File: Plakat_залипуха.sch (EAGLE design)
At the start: 25 parts, among them X1 USB-MICROB

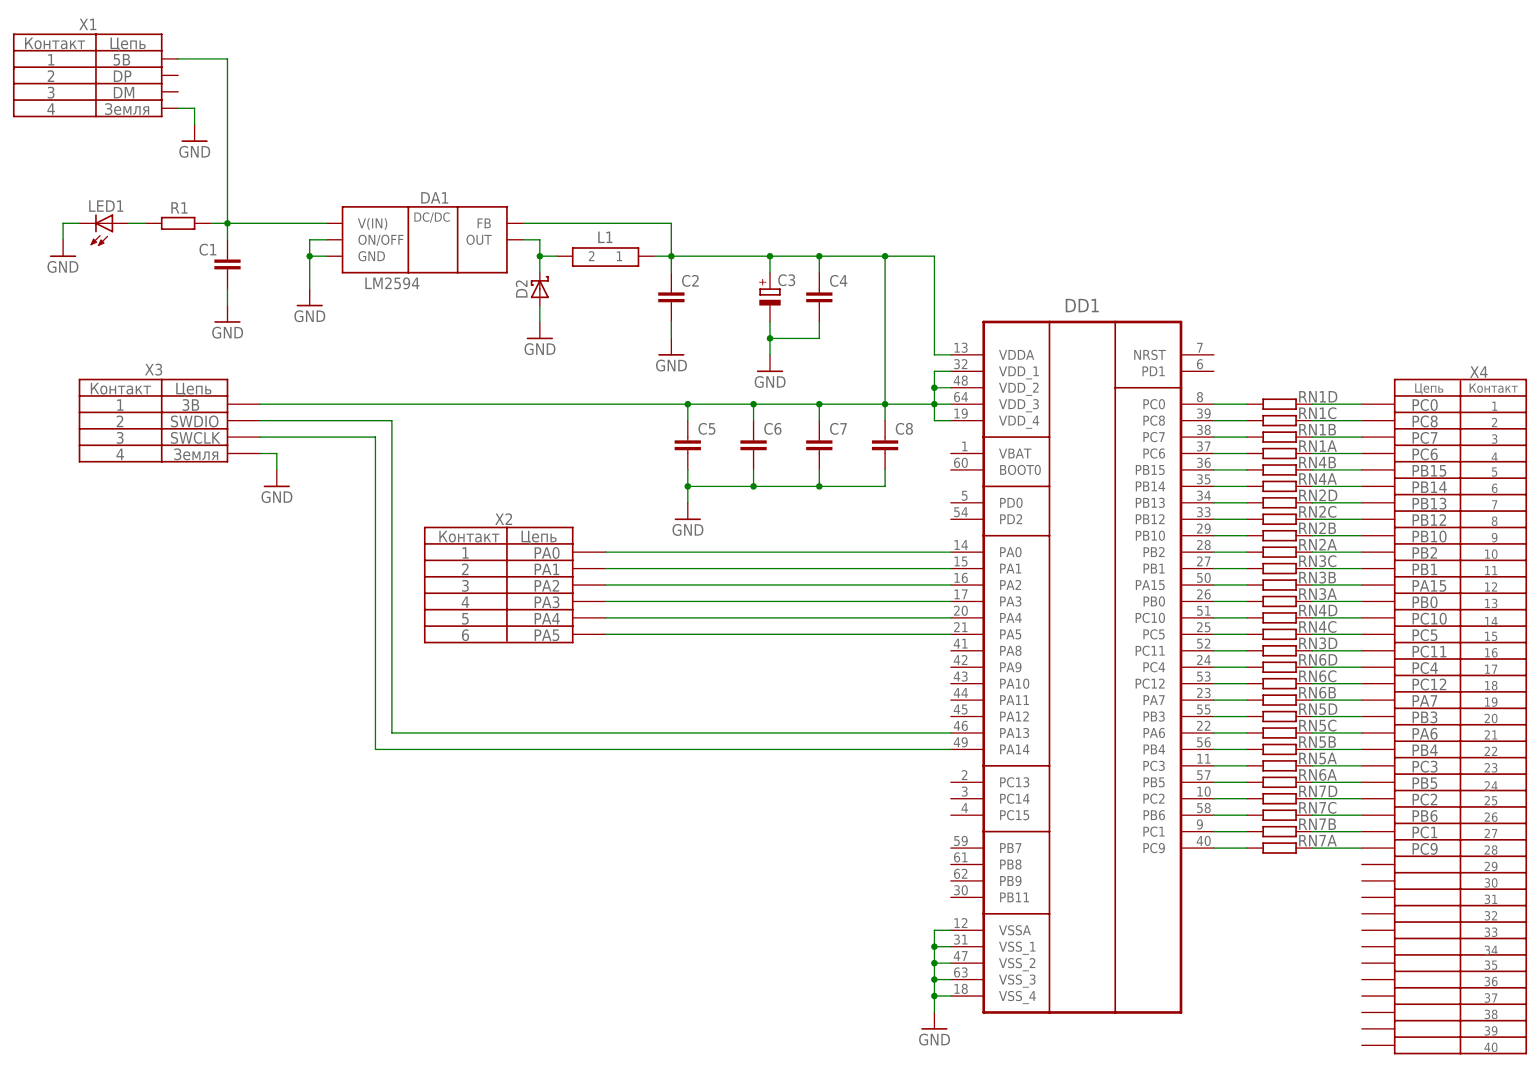
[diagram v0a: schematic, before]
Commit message: Edited plakat_залипуха
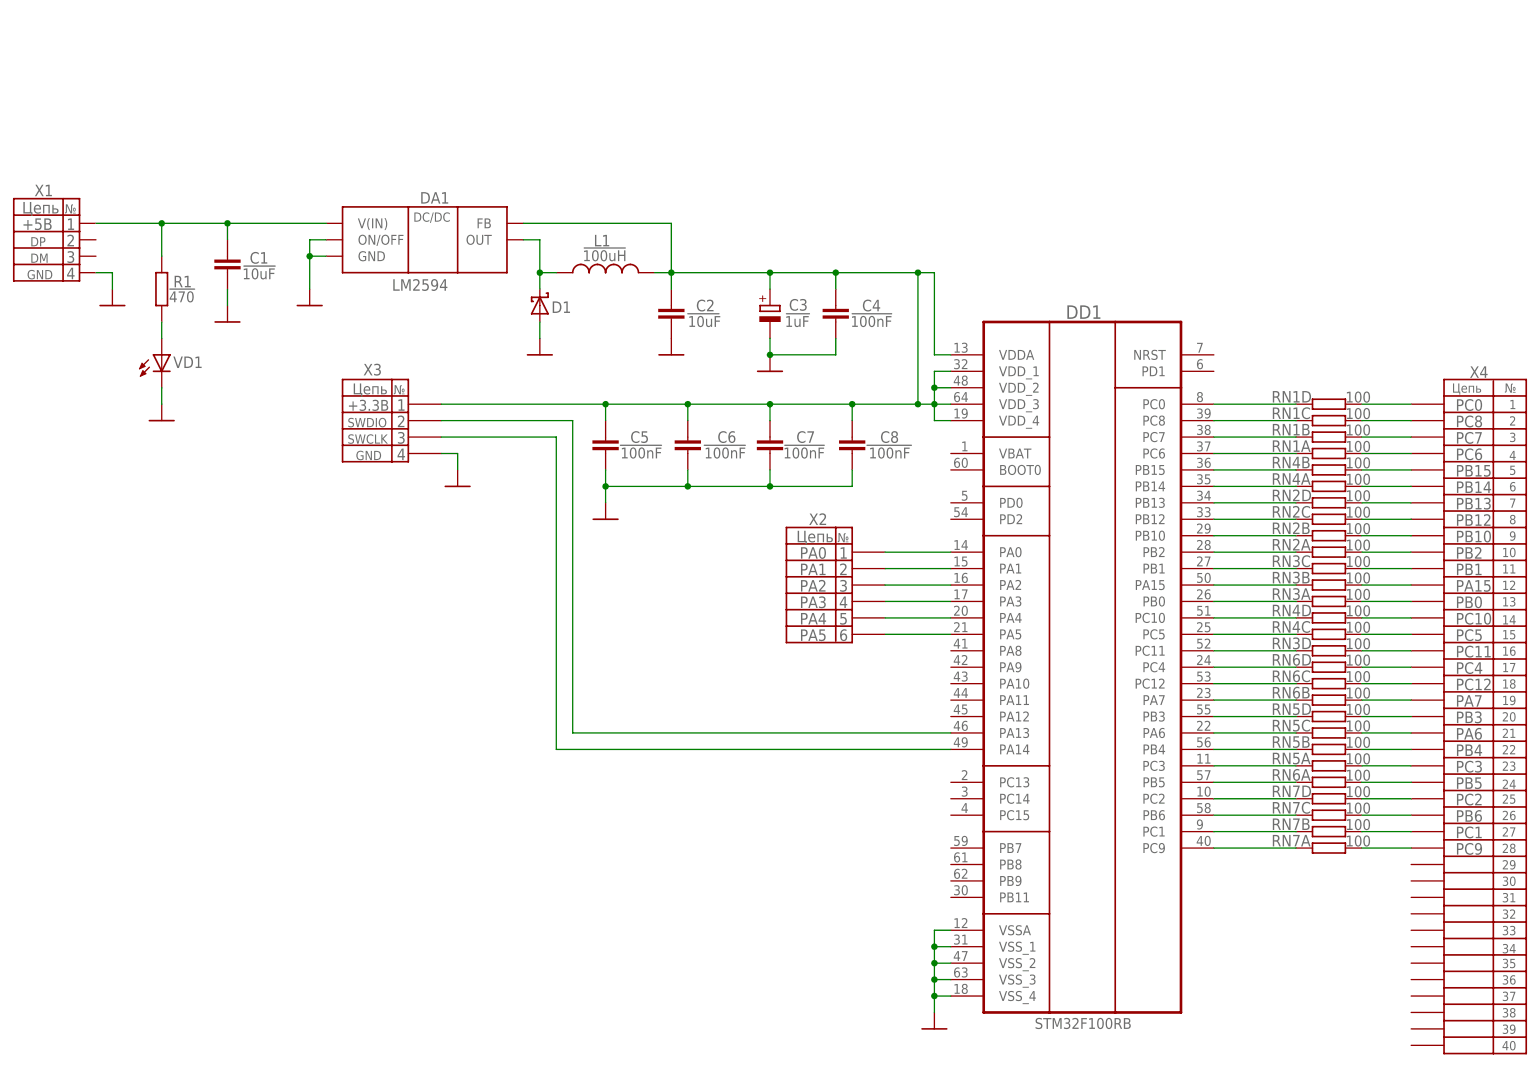
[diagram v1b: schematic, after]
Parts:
- removed D2: 1N5819-T, diode:1N5819-T
- removed LED1: (no value), eagle-ltspice:LED_E
- added D1: 1N5819-T, diode:1N5819-T
- added VD1: (no value), eagle-ltspice:LED_E
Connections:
- net GND: now also D1.A, VD1.C; no longer D2.A, LED1.C
- net N$2: now also D1.C; no longer D2.C
- net N$4: now also VD1.A; no longer LED1.A
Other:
- note added: "+3.3В"
- note added: "+5В"
- note added: "100"
- note added: "100nF"
- note added: "100uH"
- note added: "10uF"
- note added: "1uF"
- note added: "470"
- note added: "GND"
- note added: "STM32F100RB"
- note added: "№"
- note removed: "3В"
- note removed: "5В"
- note removed: "Земля"
- note removed: "Контакт"
- moved on the sheet: C2, C3, C4, C5, C6, C7, C8, R1, RN1A, RN1B, RN1C, RN1D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
